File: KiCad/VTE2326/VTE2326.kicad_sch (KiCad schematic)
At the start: 24 parts, among them J1 Power, J3 Programer, M1 Motor_DC, SW1 Reset, SW2 Mode, U1 AMS1117-3.3, U2 ESP-12E, U3 NPK, U4 L293D, U5 AMS1117-5.0

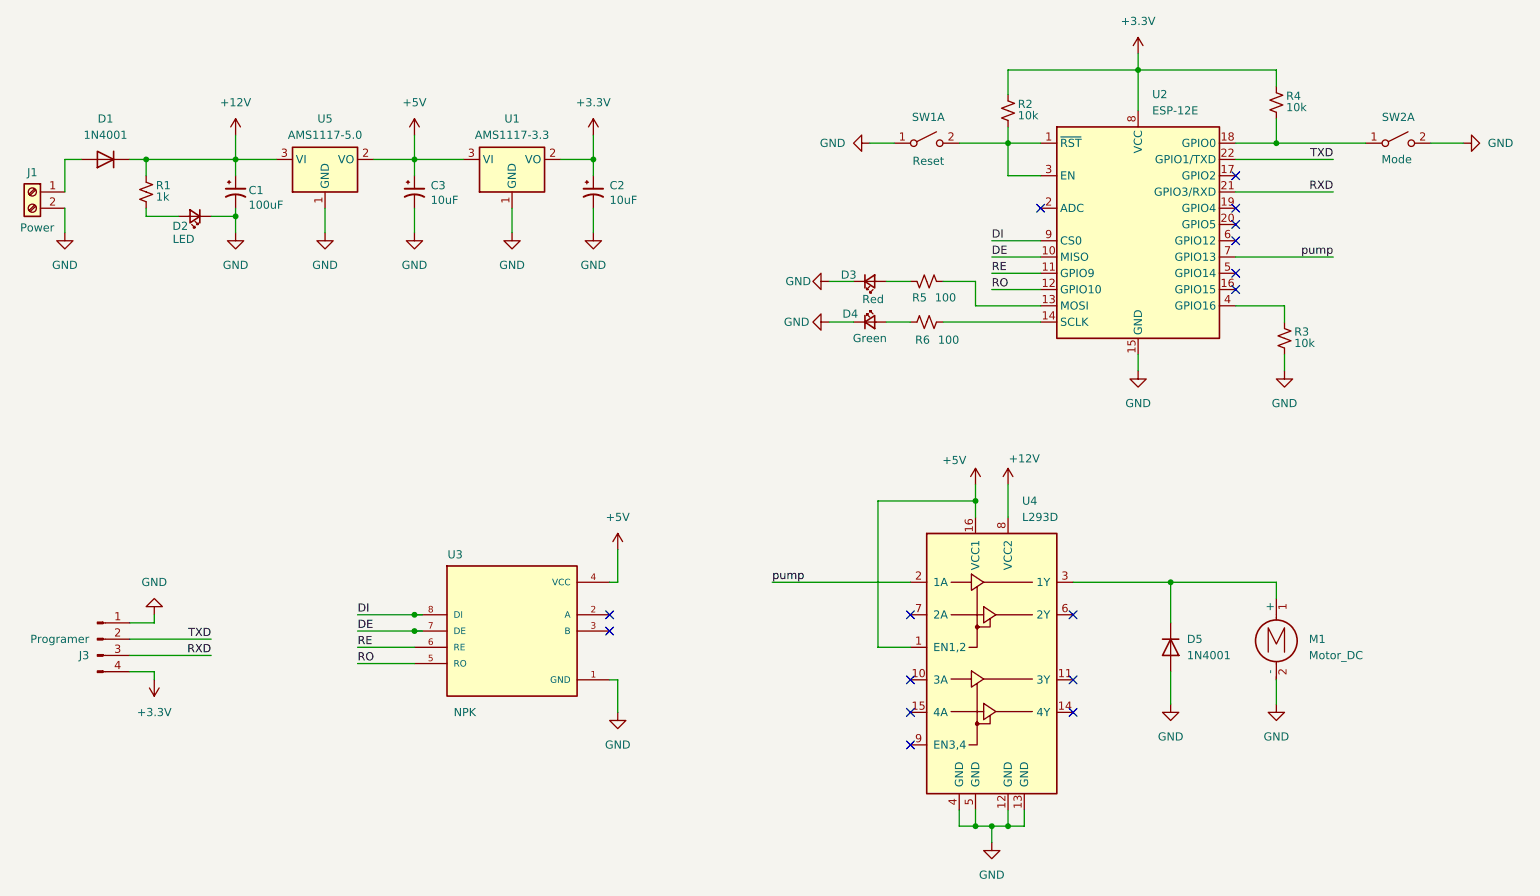
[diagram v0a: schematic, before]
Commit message: Updates
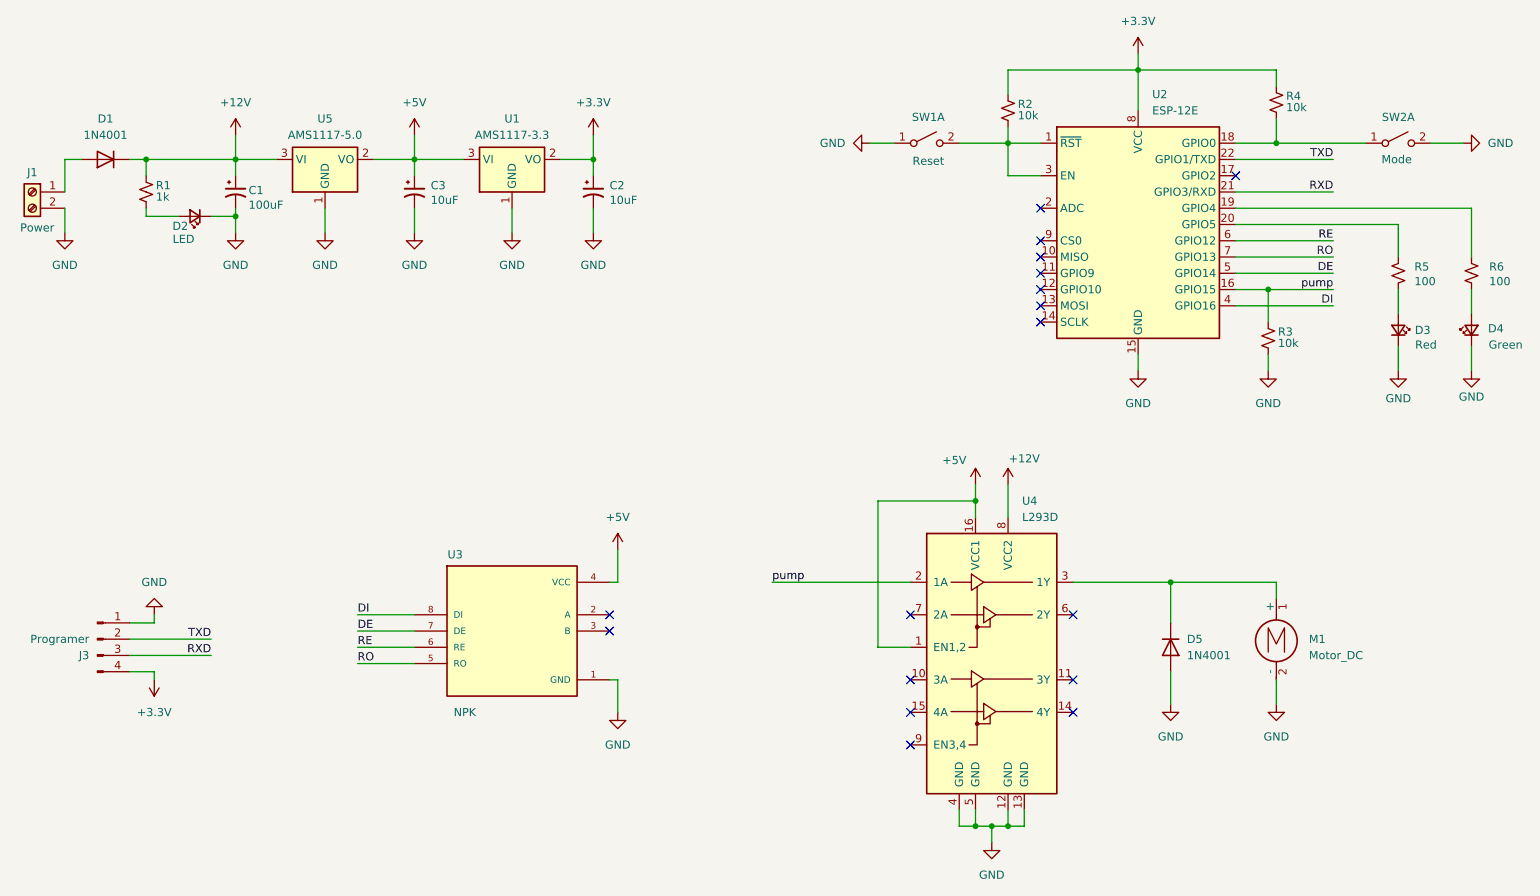
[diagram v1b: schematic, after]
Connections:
- net DE: now also U2.5 (GPIO14); no longer U2.10 (MISO)
- net DI: now also U2.4 (GPIO16); no longer U2.9 (CS0)
- net RE: now also U2.6 (GPIO12); no longer U2.11 (GPIO9)
- net RO: now also U2.7 (GPIO13); no longer U2.12 (GPIO10)
- net pump: now also R3.1, U2.16 (GPIO15); no longer U2.7 (GPIO13)
- net at R5.1: now also U2.20 (GPIO5); no longer U2.13 (MOSI)
- net at U2.14 (SCLK): no longer R6.2
- net at U2.19 (GPIO4): now also R6.2
- no-connect marks 16 -> 17
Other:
- moved on the sheet: D3, D4, R3, R5, R6
